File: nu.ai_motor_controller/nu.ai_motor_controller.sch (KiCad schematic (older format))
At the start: 0 parts

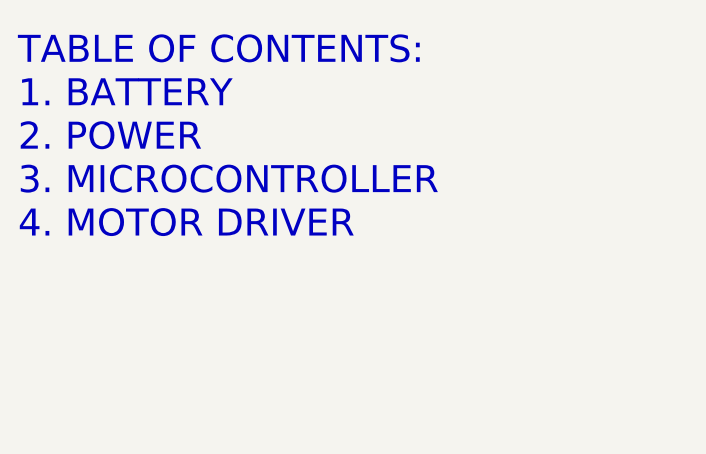
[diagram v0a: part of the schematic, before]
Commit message: automated commit
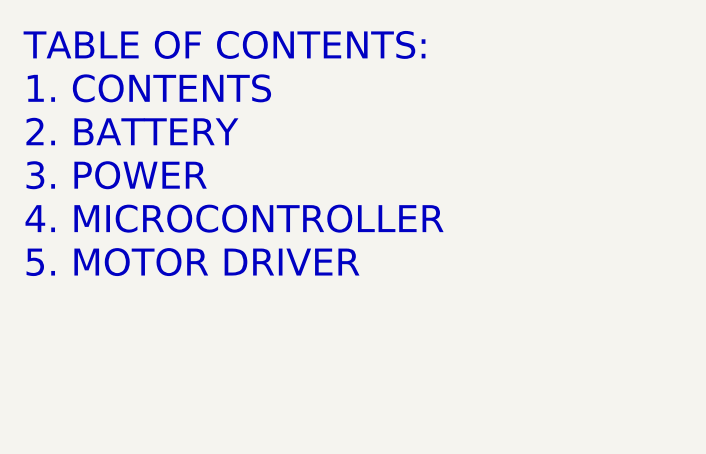
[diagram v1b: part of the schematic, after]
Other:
- note added: "TABLE OF CONTENTS:\n1. CONTENTS\n2. BATTERY\n3. POWER\n4. MICROCONTROLLER\n5. MOTOR DRIVER"
- note removed: "TABLE OF CONTENTS:\n1. BATTERY\n2. POWER\n3. MICROCONTROLLER\n4. MOTOR DRIVER"
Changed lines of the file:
@@
 Text Notes 6450 1000 0    118  ~ 0
 TODO:\nADD MOUNTING HOLES
-Text Notes 625  1550 0    118  ~ 0
-TABLE OF CONTENTS:\n1. BATTERY\n2. POWER\n3. MICROCONTROLLER\n4. MOTOR DRIVER
+Text Notes 650  1725 0    118  ~ 0
+TABLE OF CONTENTS:\n1. CONTENTS\n2. BATTERY\n3. POWER\n4. MICROCONTROLLER\n5. MOTOR DRIVER
 Text Notes 3775 825  0    118  ~ 0
 NOTES:
